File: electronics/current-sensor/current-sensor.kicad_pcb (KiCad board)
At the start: 2 copper layers, 8 parts, among them J1 PWR, J2 Out sensor, U1 LM358

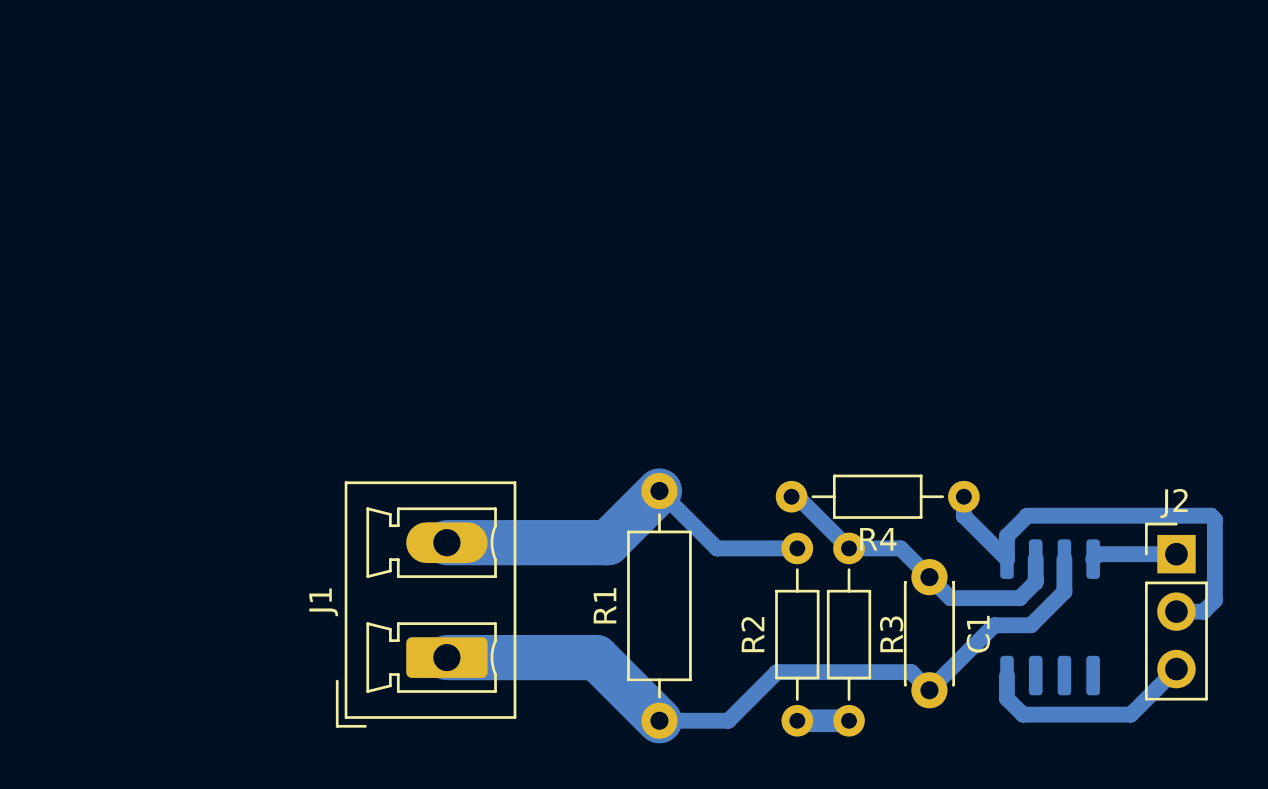
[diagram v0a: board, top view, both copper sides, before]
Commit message: Double sensor
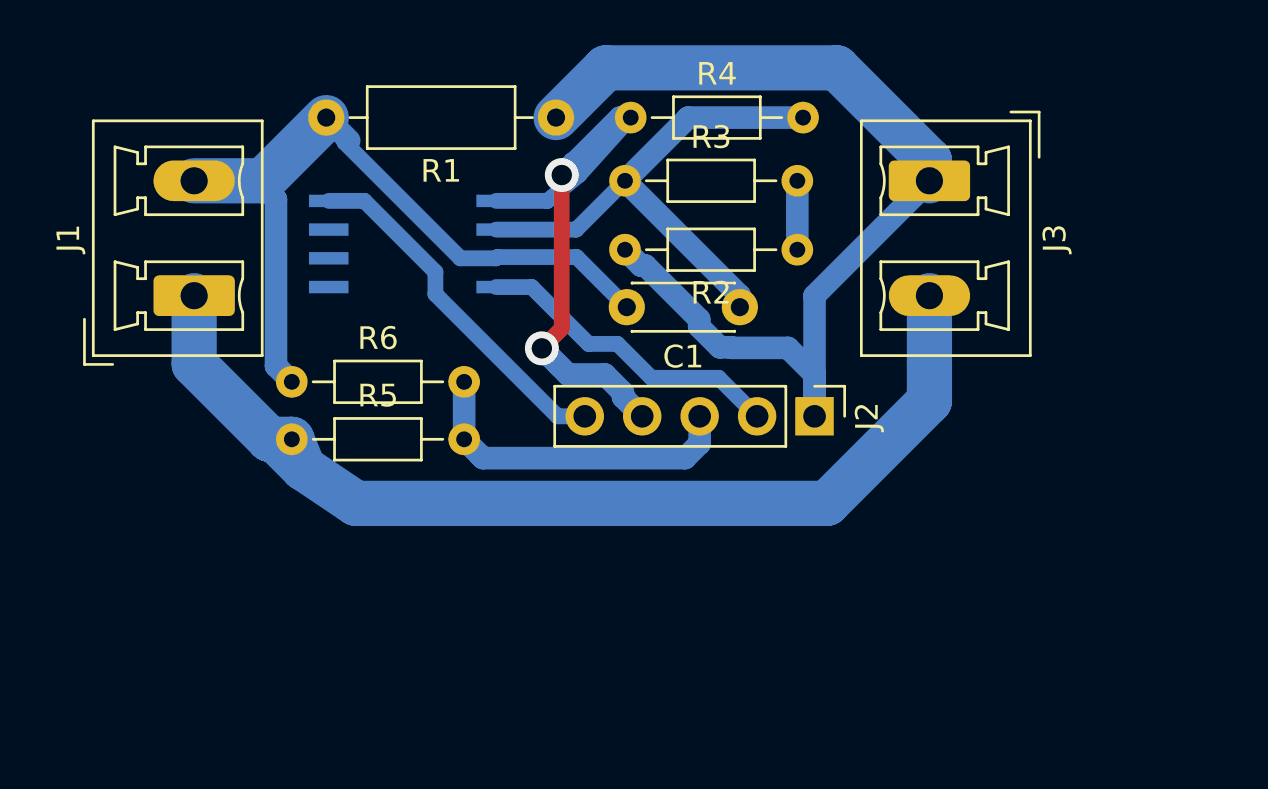
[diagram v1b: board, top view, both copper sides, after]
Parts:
- added J3: PWROUT, Connector_Phoenix_MC_HighVoltage:PhoenixContact_MCV_1,5_2-G-5.08_1x02_P5.08mm_Vertical, F.Cu at (117.9, 51.3)
- added R5: 10k, Resistor_THT:R_Axial_DIN0204_L3.6mm_D1.6mm_P7.62mm_Horizontal, F.Cu at (89.7, 62.7)
- added R6: 1k, Resistor_THT:R_Axial_DIN0204_L3.6mm_D1.6mm_P7.62mm_Horizontal, F.Cu at (89.7, 60.2)
- J1: value PWR -> PWRIN
- J2: footprint Connector_PinHeader_2.54mm:PinHeader_1x03_P2.54mm_Vertical -> Connector_PinHeader_2.54mm:PinHeader_1x05_P2.54mm_Vertical
- U1: footprint Package_SO:SO-8_3.9x4.9mm_P1.27mm -> Package_SO:SO-8_5.3x6.2mm_P1.27mm
- moved U1 32.7 mm to (95.0, 54.1), turned to 180 degrees
- moved R1 27.1 mm to (101.3, 48.5), turned to 180 degrees
- moved R4 22.3 mm to (104.6, 48.5), turned to 0 degrees
- moved R2 20.8 mm to (112.0, 54.4), turned to 180 degrees
- moved J1 19.5 mm to (85.3, 56.4)
- moved R3 19.0 mm to (104.4, 51.3), turned to 0 degrees
- moved J2 17.1 mm to (112.8, 61.7), turned to 270 degrees
- moved C1 14.6 mm to (109.5, 56.9), turned to 180 degrees
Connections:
- J1 pad 1: Net-(C1-Pad2) -> Net-(J1-Pad1)
- J1 pad 2: Net-(J1-Pad2) -> Net-(C1-Pad2)
- J2 pad 3: Net-(J2-Pad3) -> VSENS
- R1 pad 1: Net-(C1-Pad2) -> Net-(J2-Pad1)
- R1 pad 2: Net-(J1-Pad2) -> Net-(C1-Pad2)
- R2 pad 2: Net-(J1-Pad2) -> Net-(J2-Pad1)
- R4 pad 1: Net-(J2-Pad2) -> Net-(J2-Pad4)
- U1 pad 1: Net-(J2-Pad2) -> Net-(J2-Pad4)
- U1 pad 4: Net-(J2-Pad1) -> Net-(J2-Pad2)
- U1 pad 8: Net-(J2-Pad3) -> Net-(J2-Pad5)
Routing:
- net Net-(J1-Pad1): track 0.00 -> 46.8 mm
- net Net-(J2-Pad1): track 3.77 -> 45.2 mm
- net Net-(J2-Pad4): track 0.00 -> 26.2 mm, vias 0 -> 2
- net Net-(J1-Pad2): track 17.5 -> 0.00 mm
- net Net-(J2-Pad5): track 0.00 -> 15.8 mm
- net VSENS: track 0.00 -> 14.8 mm
- net Net-(J2-Pad3): track 9.64 -> 0.00 mm
- net Net-(C1-Pad1): track 14.0 -> 23.3 mm
- net Net-(J2-Pad2): track 19.7 -> 13.9 mm
- net Net-(C1-Pad2): track 32.9 -> 36.9 mm
- net Net-(R2-Pad1): track 2.29 -> 3.05 mm
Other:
- net class Default: trace_width 0.7 -> 2; via_dia 0.8 -> 1.5; via_drill 0.4 -> 0.9
